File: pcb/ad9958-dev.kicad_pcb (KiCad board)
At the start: 4 copper layers, 40 x 32 mm, 88 parts, among them J2 5V, J3 OUT0, J4 OUT1, J5 HEAD-M10X2, U1 LM1117-FIXED-SOT223, U2 LMH6714, U3 AD9958, U4 LMH6714, X1 25 MHz

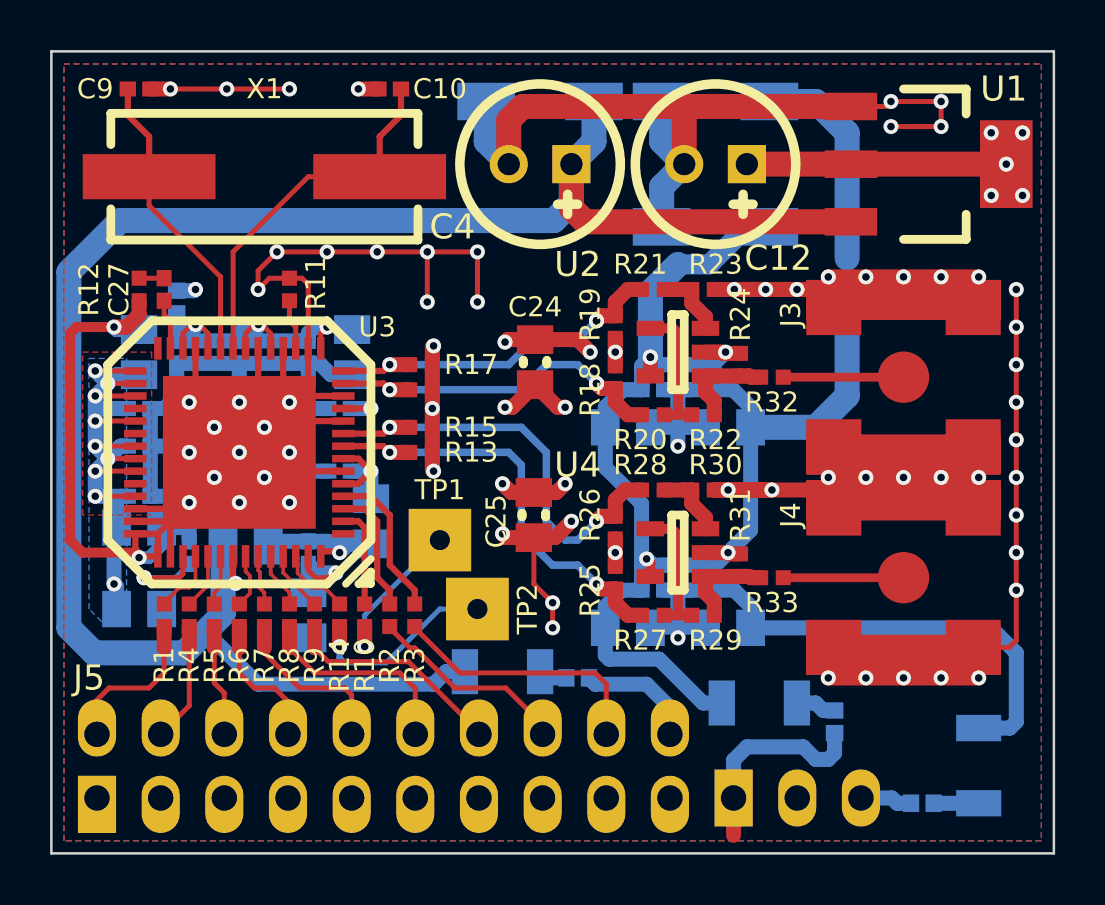
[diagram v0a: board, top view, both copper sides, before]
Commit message: Schematic touchups
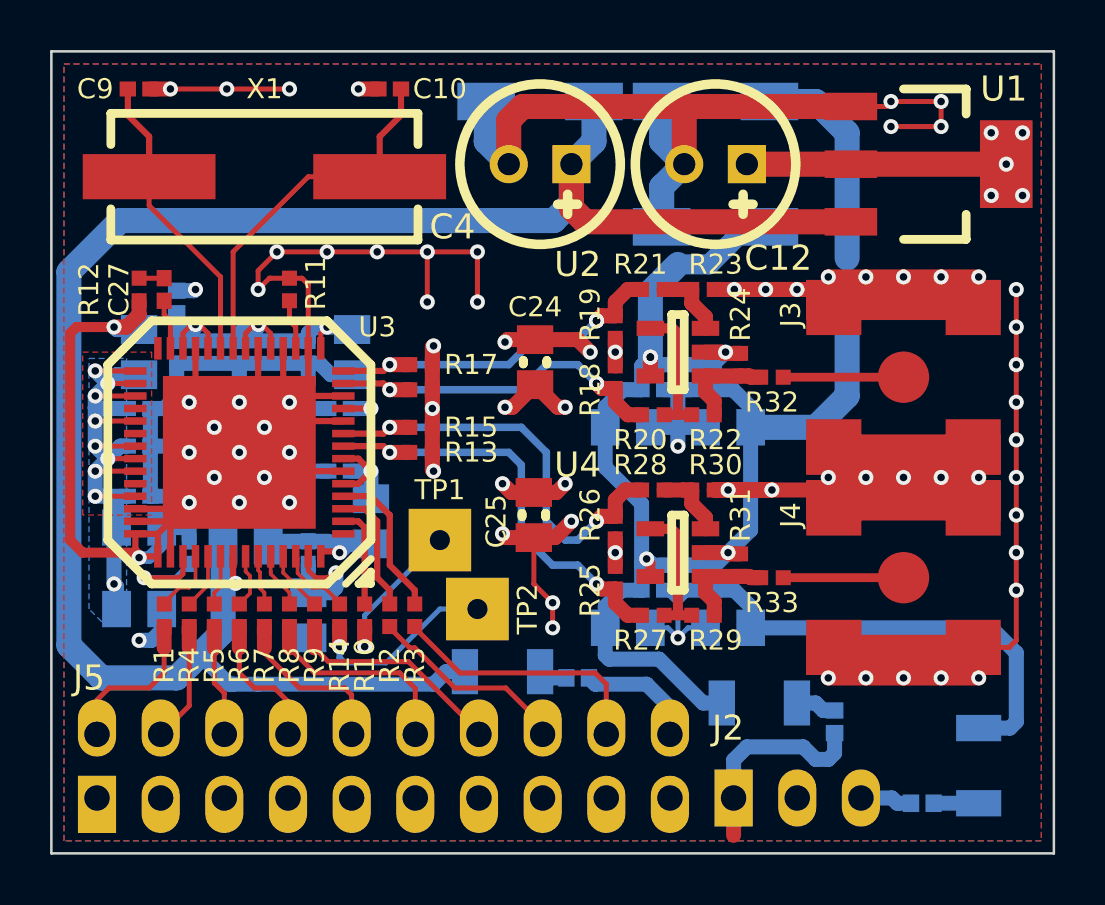
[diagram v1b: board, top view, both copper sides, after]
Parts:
- C30, C31, C35, C36: value 10n -> 1n
- J2: moved to F.Cu
- J5: value HEAD-M10X2 -> INTERFACE
- U1: value LM1117-FIXED-SOT223 -> LM1117-1v8-SOT223
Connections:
- net /+1v8A renamed +1.8A
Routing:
- net GND: track 394.5 -> 398.1 mm, vias 69 -> 70
- net +1.8: track 56.8 -> 58.7 mm, vias 9 -> 8
- net +3.3: track 75.7 -> 77.4 mm
- net +1.8A: track 63.5 -> 64.6 mm

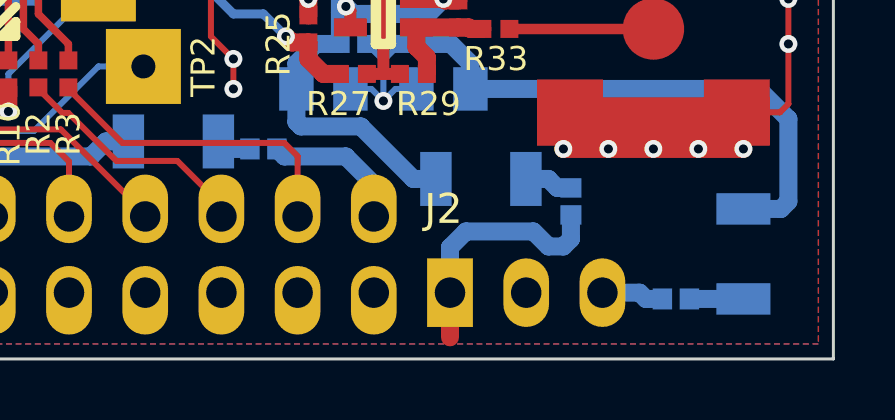
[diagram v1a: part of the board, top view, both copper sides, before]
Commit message: PCB fixes
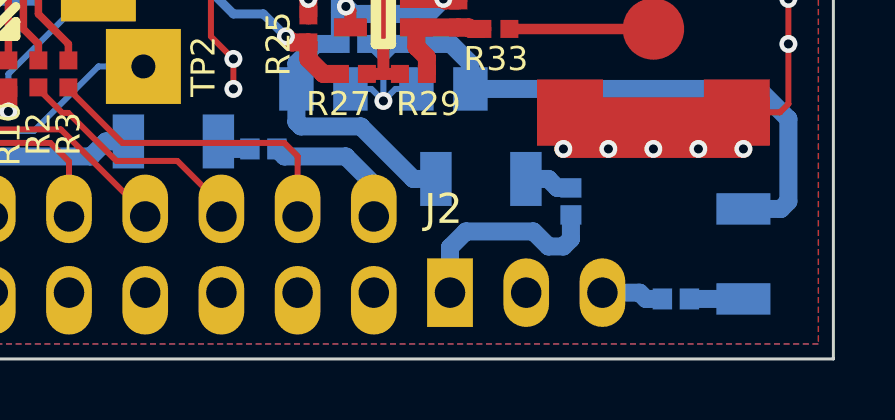
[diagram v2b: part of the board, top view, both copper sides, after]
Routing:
- net Net-(E2-Pad2): track 8.36 -> 6.87 mm
